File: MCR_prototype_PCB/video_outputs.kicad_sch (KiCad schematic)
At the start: 25 parts, among them J1-VGAOut1 DE15_Socket_HighDensity, J2_RGBS_Out1 Conn_01x09_Pin, U12 THS7374, U13 THS7374

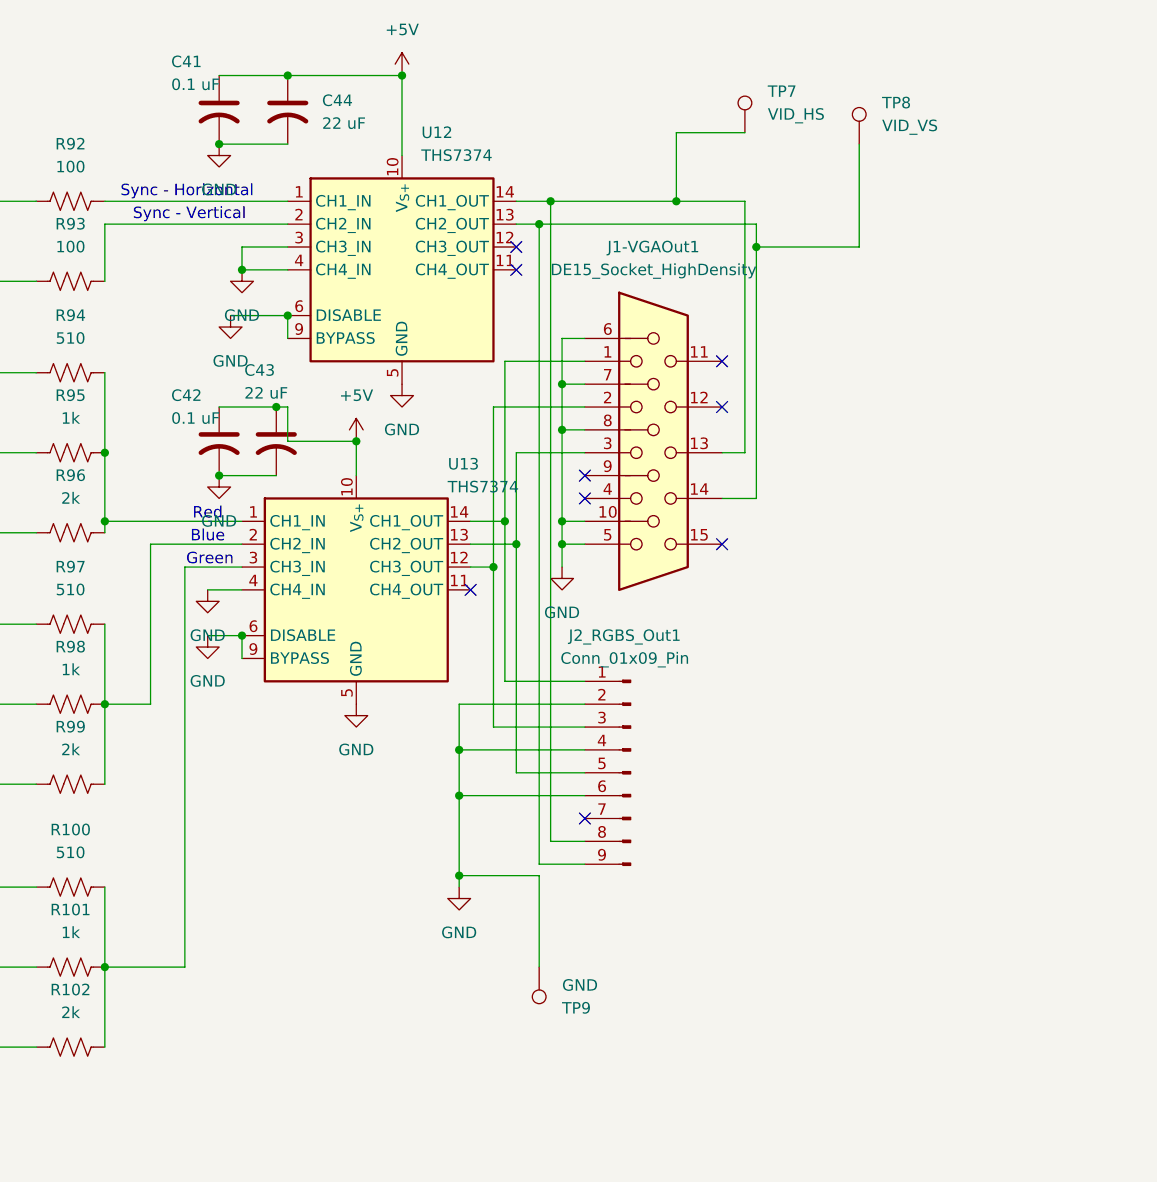
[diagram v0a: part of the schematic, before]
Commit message: Add files via upload
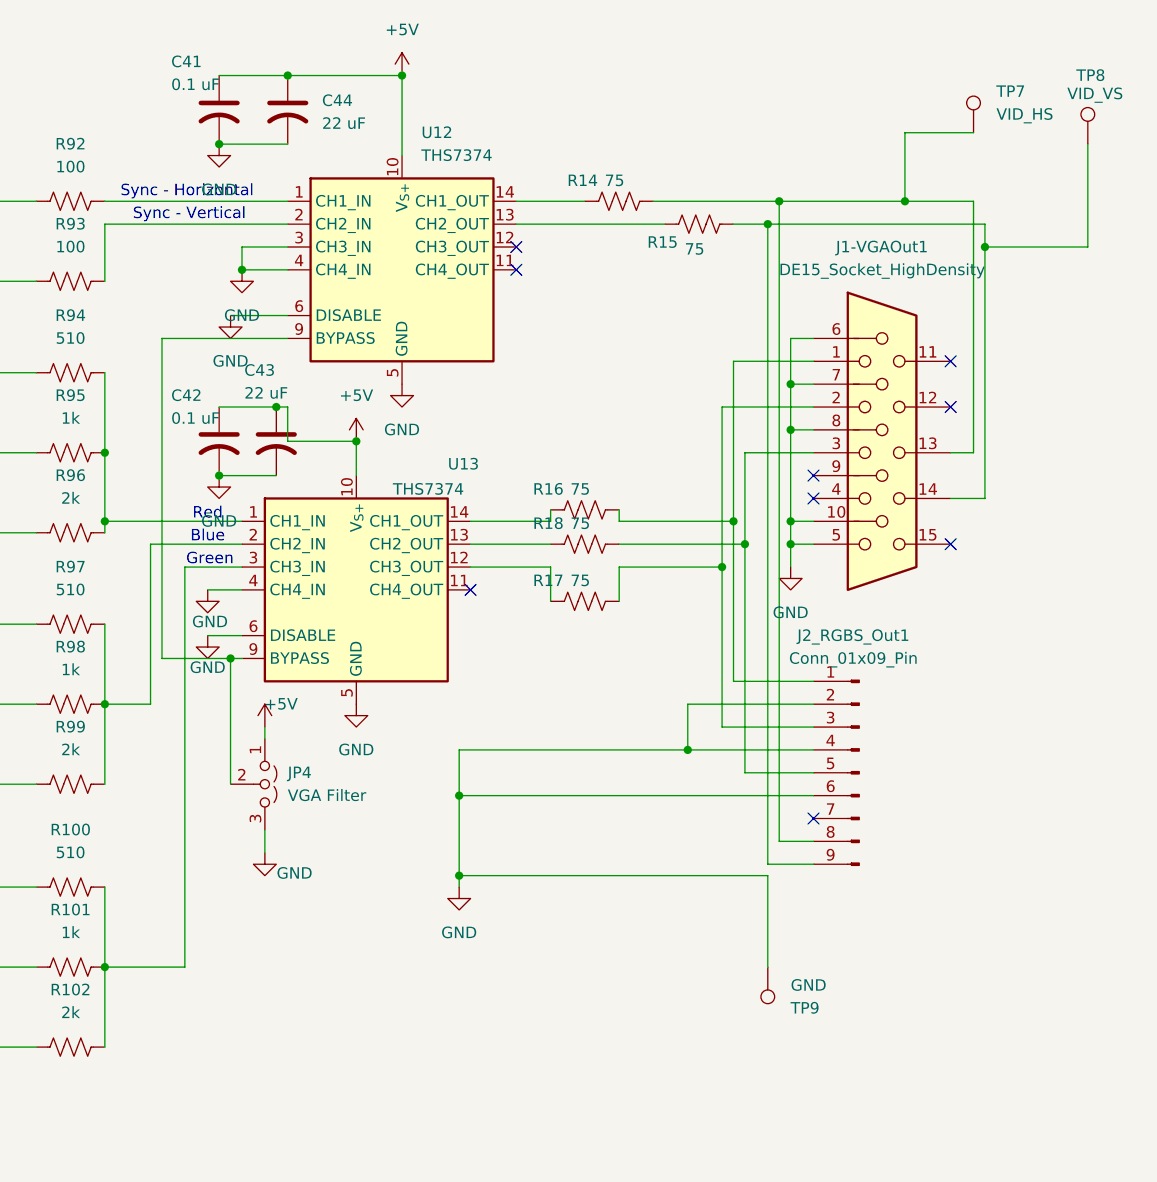
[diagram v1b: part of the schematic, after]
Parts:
- added JP4: VGA Filter, Connector_PinHeader_2.54mm:PinHeader_1x03_P2.54mm_Vertical, symbol Jumper:Jumper_3_Open
- added R14, R15, R16, R17: 75, Resistor_SMD:R_0805_2012Metric, symbol Device:R_US
- added R18: 75, Capacitor_SMD:C_0805_2012Metric, symbol Device:R_US
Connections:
- net +5V: now also JP4.1 (A)
- net GND: now also JP4.3 (B); no longer U12.9 (BYPASS), U13.9 (BYPASS)
- net at J1-VGAOut1.1, J2_RGBS_Out1.1 (Pin_1): now also R16.2; no longer U13.14 (CH1_OUT)
- net at J1-VGAOut1.2, J2_RGBS_Out1.3 (Pin_3): now also R17.2; no longer U13.12 (CH3_OUT)
- net at J1-VGAOut1.3, J2_RGBS_Out1.5 (Pin_5): now also R18.2; no longer U13.13 (CH2_OUT)
- net at J1-VGAOut1.13, J2_RGBS_Out1.8 (Pin_8), TP7.1: now also R14.2; no longer U12.14 (CH1_OUT)
- net at J1-VGAOut1.14, J2_RGBS_Out1.9 (Pin_9), TP8.1: now also R15.2; no longer U12.13 (CH2_OUT)
- new net: JP4.2 (C), U12.9 (BYPASS), U13.9 (BYPASS)
- new net: R18.1, U13.13 (CH2_OUT)
- new net: R14.1, U12.14 (CH1_OUT)
- new net: R17.1, U13.12 (CH3_OUT)
- new net: R15.1, U12.13 (CH2_OUT)
- new net: R16.1, U13.14 (CH1_OUT)
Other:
- moved on the sheet: J1-VGAOut1, J2_RGBS_Out1, TP7, TP8, TP9
